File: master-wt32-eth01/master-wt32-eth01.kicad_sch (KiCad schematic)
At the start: 23 parts, among them J1 24V Field, J2 24V System, J3 Enable, J4 Screw_Terminal_01x03, J5 Conn_01x06_Female, J6 Conn_01x06_Female, SW1 SW_DIP_x03, U1 LM2596-Board, U2 WT32-ETH0-Board, U3 PC817

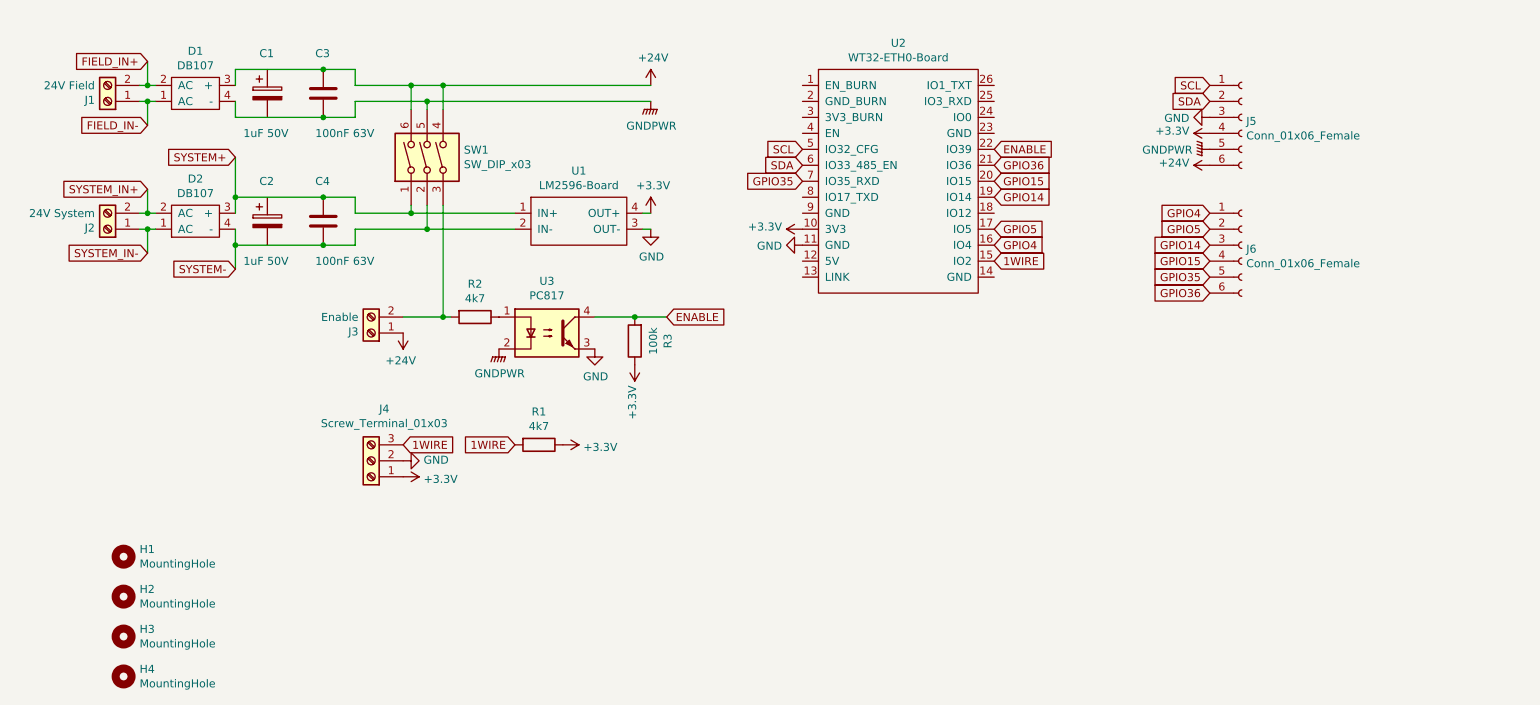
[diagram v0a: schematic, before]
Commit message: refactor power
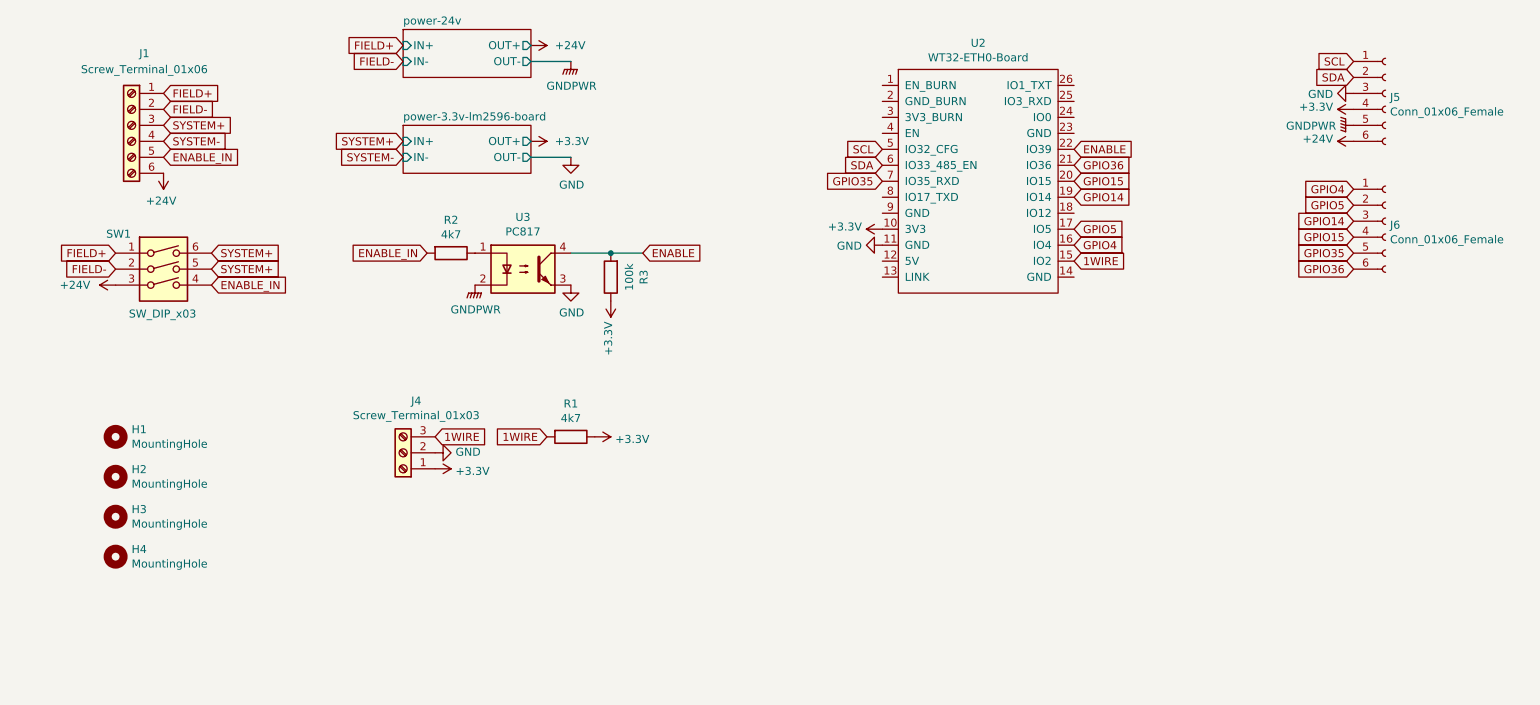
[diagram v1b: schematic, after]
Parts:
- removed C1, C2: 1uF 50V, Capacitor_THT:CP_Radial_D5.0mm_P2.50mm, symbol Device:C_Polarized
- removed C3, C4: 100nF 63V, Capacitor_THT:C_Rect_L7.0mm_W2.0mm_P5.00mm, symbol Device:C
- removed D1, D2: DB107, custom:DB107, symbol custom:DB107
- removed J1: 24V Field, TerminalBlock:TerminalBlock_bornier-2_P5.08mm, symbol Connector:Screw_Terminal_01x02
- removed J2: 24V System, TerminalBlock:TerminalBlock_bornier-2_P5.08mm, symbol Connector:Screw_Terminal_01x02
- removed J3: Enable, TerminalBlock:TerminalBlock_bornier-2_P5.08mm, symbol Connector:Screw_Terminal_01x02
- removed U1: LM2596-Board, boards:LM2596-Board, symbol boards:LM2596-Board
- added J1: Screw_Terminal_01x06, TerminalBlock:TerminalBlock_bornier-6_P5.08mm, symbol Connector:Screw_Terminal_01x06
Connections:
- net +24V: now also SW1.3, J1.6 (Pin_6); no longer SW1.4, SW1.6
- net GNDPWR: no longer SW1.5
- net SYSTEM+: now also SW1.5, SW1.6, J1.3 (Pin_3); no longer SW1.1
- net SYSTEM-: now also J1.4 (Pin_4); no longer SW1.2
- net ENABLE_IN: now reaches R2.2
- net ENABLE_IN: now also SW1.4, J1.5 (Pin_5); no longer SW1.3
- new net FIELD+: J1.1 (Pin_1), SW1.1
- new net FIELD-: J1.2 (Pin_2), SW1.2
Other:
- added sheet power-24v (../include/power-24v.kicad_sch)
- added sheet power-3.3v-lm2596-board (../include/power-3.3v-lm2596-board.kicad_sch)
- moved on the sheet: H1, H2, H3, H4, J4, J5, J6, R1, R2, R3, U2, U3
